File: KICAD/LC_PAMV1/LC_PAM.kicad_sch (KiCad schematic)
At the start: 24 parts, among them J1 Conn_01x04, J10 Conn_01x02, J11 Conn_01x02, J2 DC/DC, J3 Conn_01x24, J4 Conn_01x24, J5 Conn_01x02, J6 HPAB, J7 Conn_01x02_Pin, J8 Conn_01x06_Pin, J9 Conn_01x03, U1 teensy_Teensy4.1

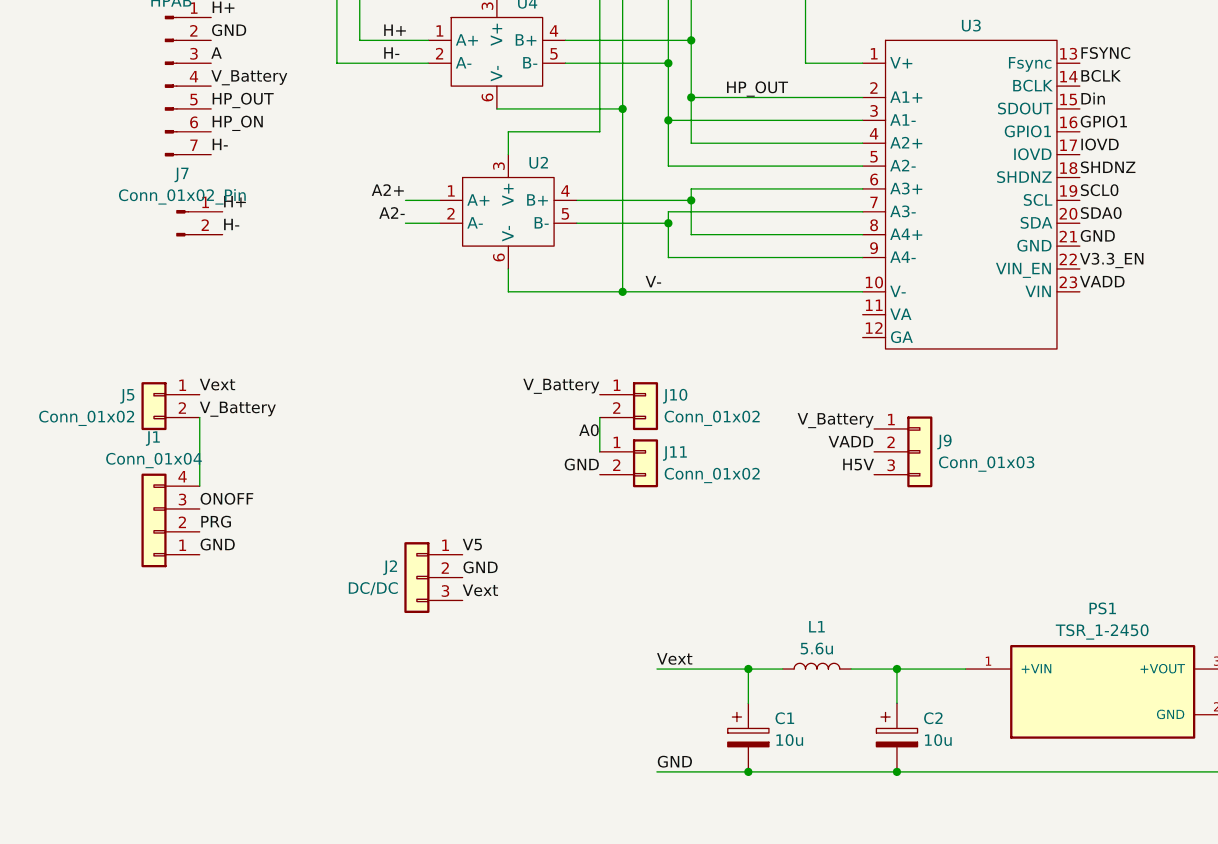
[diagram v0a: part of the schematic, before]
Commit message: v19-12-24
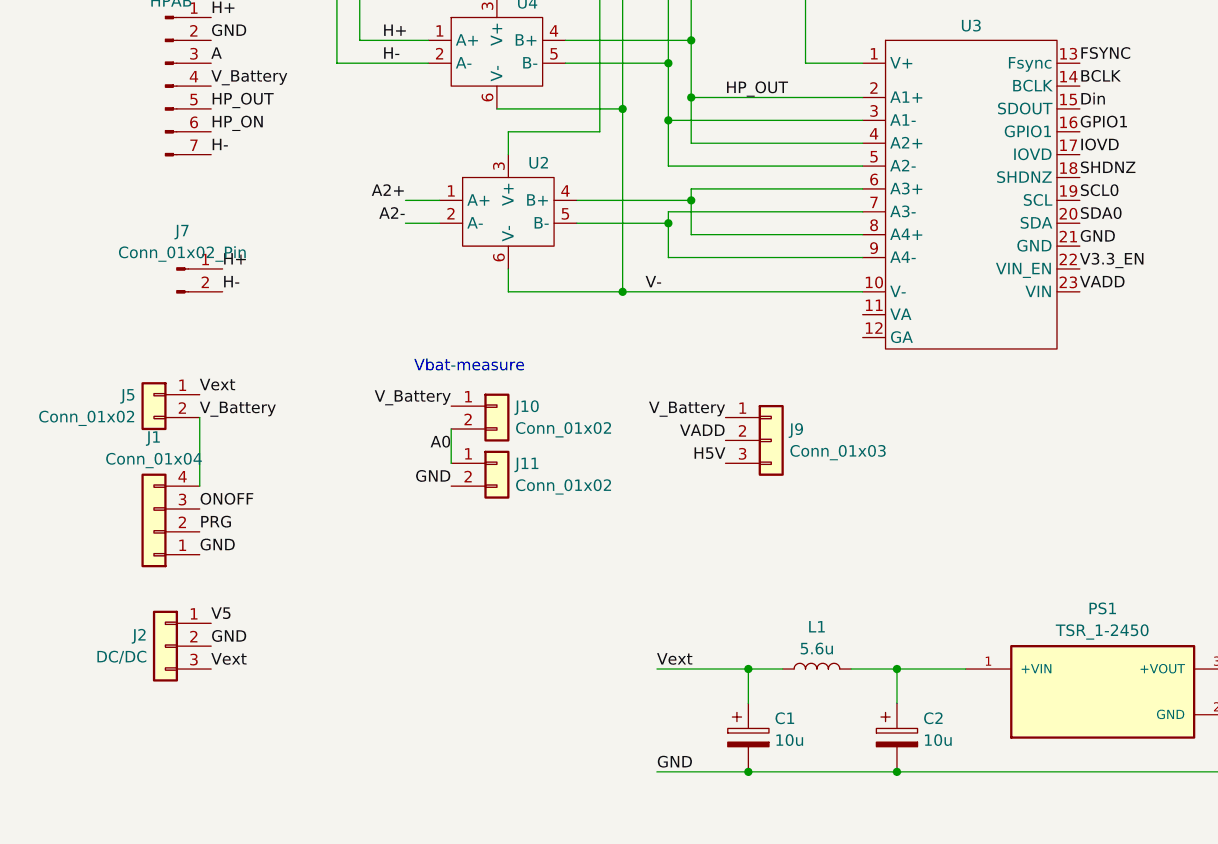
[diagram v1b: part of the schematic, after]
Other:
- note added: "Vbat-measure"
- moved on the sheet: J10, J11, J2, J7, J9
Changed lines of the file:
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@@
 	(wire
 		(pts
-			(xy 85.09 113.03) (xy 85.09 116.84)
+			(xy 68.58 114.3) (xy 68.58 118.11)
 		)
 		(stroke
@@
 		)
 	)
+	(text "Vbat-measure"
+		(exclude_from_sim no)
+		(at 70.612 107.442 0)
+		(effects
+			(font
+				(size 1.27 1.27)
+			)
+		)
+	)
 	(label "FSYNC"
 		(at 247.65 67.31 0)
@@
 	)
 	(label "GND"
-		(at 85.09 119.38 180)
+		(at 68.58 120.65 180)
 		(fields_autoplaced yes)
 		(effects
@@
 	)
 	(label "H5V"
-		(at 115.57 119.38 180)
+		(at 99.06 118.11 180)
 		(fields_autoplaced yes)
 		(effects
@@
 	)
 	(label "V_Battery"
-		(at 115.57 114.3 180)
+		(at 99.06 113.03 180)
 		(fields_autoplaced yes)
 		(effects
@@
 	)
 	(label "A0"
-		(at 85.09 115.57 180)
+		(at 68.58 116.84 180)
 		(fields_autoplaced yes)
 		(effects
@@
 	)
 	(label "V_Battery"
-		(at 85.09 110.49 180)
+		(at 68.58 111.76 180)
 		(fields_autoplaced yes)
 		(effects
@@
 	)
 	(label "GND"
-		(at 69.85 130.81 0)
+		(at 41.91 138.43 0)
 		(fields_autoplaced yes)
 		(effects
@@
 	)
 	(label "H-"
-		(at 43.18 92.71 0)
+		(at 43.18 99.06 0)
 		(fields_autoplaced yes)
 		(effects
@@
 	)
 	(label "V5"
-		(at 69.85 128.27 0)
+		(at 41.91 135.89 0)
 		(fields_autoplaced yes)
 		(effects
@@
 	)
 	(label "Vext"
-		(at 69.85 133.35 0)
+		(at 41.91 140.97 0)
 		(fields_autoplaced yes)
 		(effects
@@
 	)
 	(label "H+"
-		(at 43.18 90.17 0)
+		(at 43.18 96.52 0)
 		(fields_autoplaced yes)
 		(effects
@@
 	)
 	(label "VADD"
-		(at 115.57 116.84 180)
+		(at 99.06 115.57 180)
 		(fields_autoplaced yes)
 		(effects
@@
 	(symbol
 		(lib_id "Connector_Generic:Conn_01x02")
-		(at 90.17 116.84 0)
+		(at 73.66 118.11 0)
 		(unit 1)
 		(exclude_from_sim no)
@@
 		(fields_autoplaced yes)
 		(property "Reference" "J11"
-			(at 92.202 116.8978 0)
+			(at 75.692 118.1678 0)
 			(effects
 				(font
@@
 		)
 		(property "Value" "Conn_01x02"
-			(at 92.202 119.3221 0)
+			(at 75.692 120.5921 0)
 			(effects
 				(font
@@
 		)
 		(property "Footprint" "Resistor_THT:R_Axial_DIN0204_L3.6mm_D1.6mm_P1.90mm_Vertical"
-			(at 90.17 116.84 0)
+			(at 73.66 118.11 0)
 			(effects
 				(font
@@
 		)
 		(property "Datasheet" "~"
-			(at 90.17 116.84 0)
+			(at 73.66 118.11 0)
 			(effects
 				(font
@@
 		)
 		(property "Description" "Generic connector, single row, 01x02, script generated (kicad-library-utils/schlib/autogen/connector/)"
-			(at 90.17 116.84 0)
+			(at 73.66 118.11 0)
 			(effects
 				(font
@@
 	(symbol
 		(lib_id "Connector_Generic:Conn_01x03")
-		(at 64.77 130.81 0)
+		(at 36.83 138.43 0)
 		(mirror y)
 		(unit 1)
@@
 		(dnp no)
 		(property "Reference" "J2"
-			(at 62.738 129.5978 0)
+			(at 34.798 137.2178 0)
 			(effects
 				(font
@@
 		)
 		(property "Value" "DC/DC"
-			(at 62.738 132.0221 0)
+			(at 34.798 139.6421 0)
 			(effects
 				(font
@@
 		)
 		(property "Footprint" "Connector_PinHeader_2.54mm:PinHeader_1x03_P2.54mm_Vertical"
-			(at 64.77 130.81 0)
+			(at 36.83 138.43 0)
 			(effects
 				(font
@@
 		)
 		(property "Datasheet" "~"
-			(at 64.77 130.81 0)
+			(at 36.83 138.43 0)
 			(effects
 				(font
@@
 		)
 		(property "Description" "Generic connector, single row, 01x03, script generated (kicad-library-utils/schlib/autogen/connector/)"
-			(at 64.77 130.81 0)
+			(at 36.83 138.43 0)
 			(effects
 				(font
@@
 	(symbol
 		(lib_id "Connector:Conn_01x02_Pin")
-		(at 38.1 90.17 0)
+		(at 38.1 96.52 0)
 		(unit 1)
 		(exclude_from_sim no)
@@
 		(fields_autoplaced yes)
 		(property "Reference" "J7"
-			(at 38.735 85.9493 0)
+			(at 38.735 92.2993 0)
 			(effects
 				(font
@@
 		)
 		(property "Value" "Conn_01x02_Pin"
-			(at 38.735 88.3736 0)
+			(at 38.735 94.7236 0)
 			(effects
 				(font
@@
 		)
 		(property "Footprint" "Connector_Molex:Molex_PicoBlade_53047-0210_1x02_P1.25mm_Vertical"
-			(at 38.1 90.17 0)
+			(at 38.1 96.52 0)
 			(effects
 				(font
@@
 		)
 		(property "Datasheet" "~"
-			(at 38.1 90.17 0)
+			(at 38.1 96.52 0)
 			(effects
 				(font
@@
 		)
 		(property "Description" "Generic connector, single row, 01x02, script generated"
-			(at 38.1 90.17 0)
+			(at 38.1 96.52 0)
 			(effects
 				(font
@@
 	(symbol
 		(lib_id "Connector_Generic:Conn_01x03")
-		(at 120.65 116.84 0)
+		(at 104.14 115.57 0)
 		(unit 1)
 		(exclude_from_sim no)
@@
 		(fields_autoplaced yes)
 		(property "Reference" "J9"
-			(at 122.682 115.6278 0)
+			(at 106.172 114.3578 0)
 			(effects
 				(font
@@
 		)
 		(property "Value" "Conn_01x03"
-			(at 122.682 118.0521 0)
+			(at 106.172 116.7821 0)
 			(effects
 				(font
@@
 		)
 		(property "Footprint" "Connector_Wire:SolderWire-0.1sqmm_1x03_P3.6mm_D0.4mm_OD1mm"
-			(at 120.65 116.84 0)
+			(at 104.14 115.57 0)
 			(effects
 				(font
@@
 		)
 		(property "Datasheet" "~"
-			(at 120.65 116.84 0)
+			(at 104.14 115.57 0)
 			(effects
 				(font
@@
 		)
 		(property "Description" "Generic connector, single row, 01x03, script generated (kicad-library-utils/schlib/autogen/connector/)"
-			(at 120.65 116.84 0)
+			(at 104.14 115.57 0)
 			(effects
 				(font
@@
 	(symbol
 		(lib_id "Connector_Generic:Conn_01x02")
-		(at 90.17 110.49 0)
+		(at 73.66 111.76 0)
 		(unit 1)
 		(exclude_from_sim no)
@@
 		(fields_autoplaced yes)
 		(property "Reference" "J10"
-			(at 92.202 110.5478 0)
+			(at 75.692 111.8178 0)
 			(effects
 				(font
@@
 		)
 		(property "Value" "Conn_01x02"
-			(at 92.202 112.9721 0)
+			(at 75.692 114.2421 0)
 			(effects
 				(font
@@
 		)
 		(property "Footprint" "Resistor_THT:R_Axial_DIN0204_L3.6mm_D1.6mm_P1.90mm_Vertical"
-			(at 90.17 110.49 0)
+			(at 73.66 111.76 0)
 			(effects
 				(font
@@
 		)
 		(property "Datasheet" "~"
-			(at 90.17 110.49 0)
+			(at 73.66 111.76 0)
 			(effects
 				(font
@@
 		)
 		(property "Description" "Generic connector, single row, 01x02, script generated (kicad-library-utils/schlib/autogen/connector/)"
-			(at 90.17 110.49 0)
+			(at 73.66 111.76 0)
 			(effects
 				(font
